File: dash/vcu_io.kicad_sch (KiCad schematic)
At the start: 56 parts, among them J3 M80-5102042, Q2 XP262N7002TR-G, Q3 XP262N7002TR-G, Q4 XP262N7002TR-G, Q5 XP262N7002TR-G, U30 TCAN3404-Q1, U42 TCAN3404-Q1

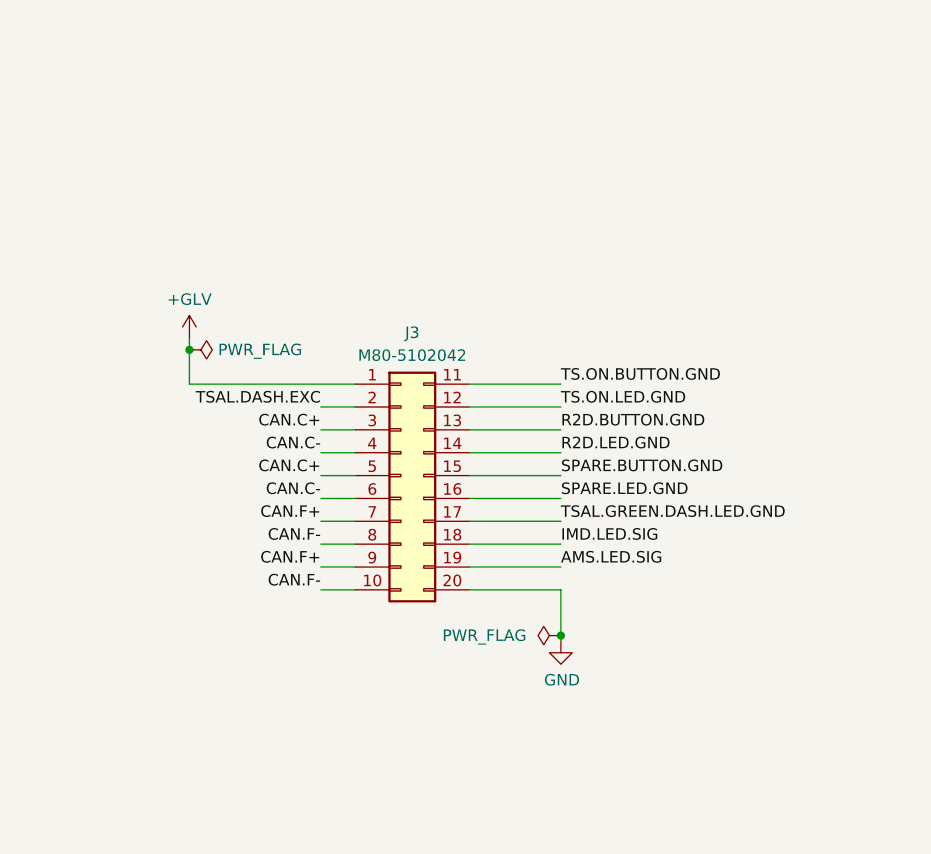
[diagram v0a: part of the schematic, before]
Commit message: Changed Inductors
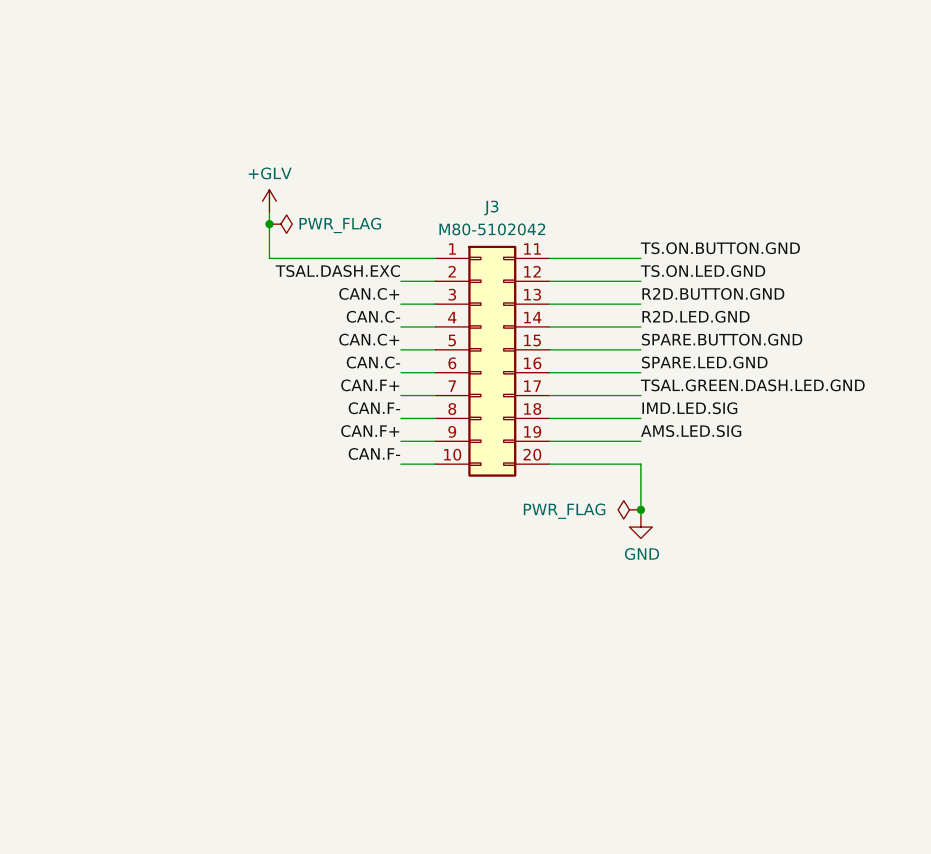
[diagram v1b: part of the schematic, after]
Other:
- moved on the sheet: J3

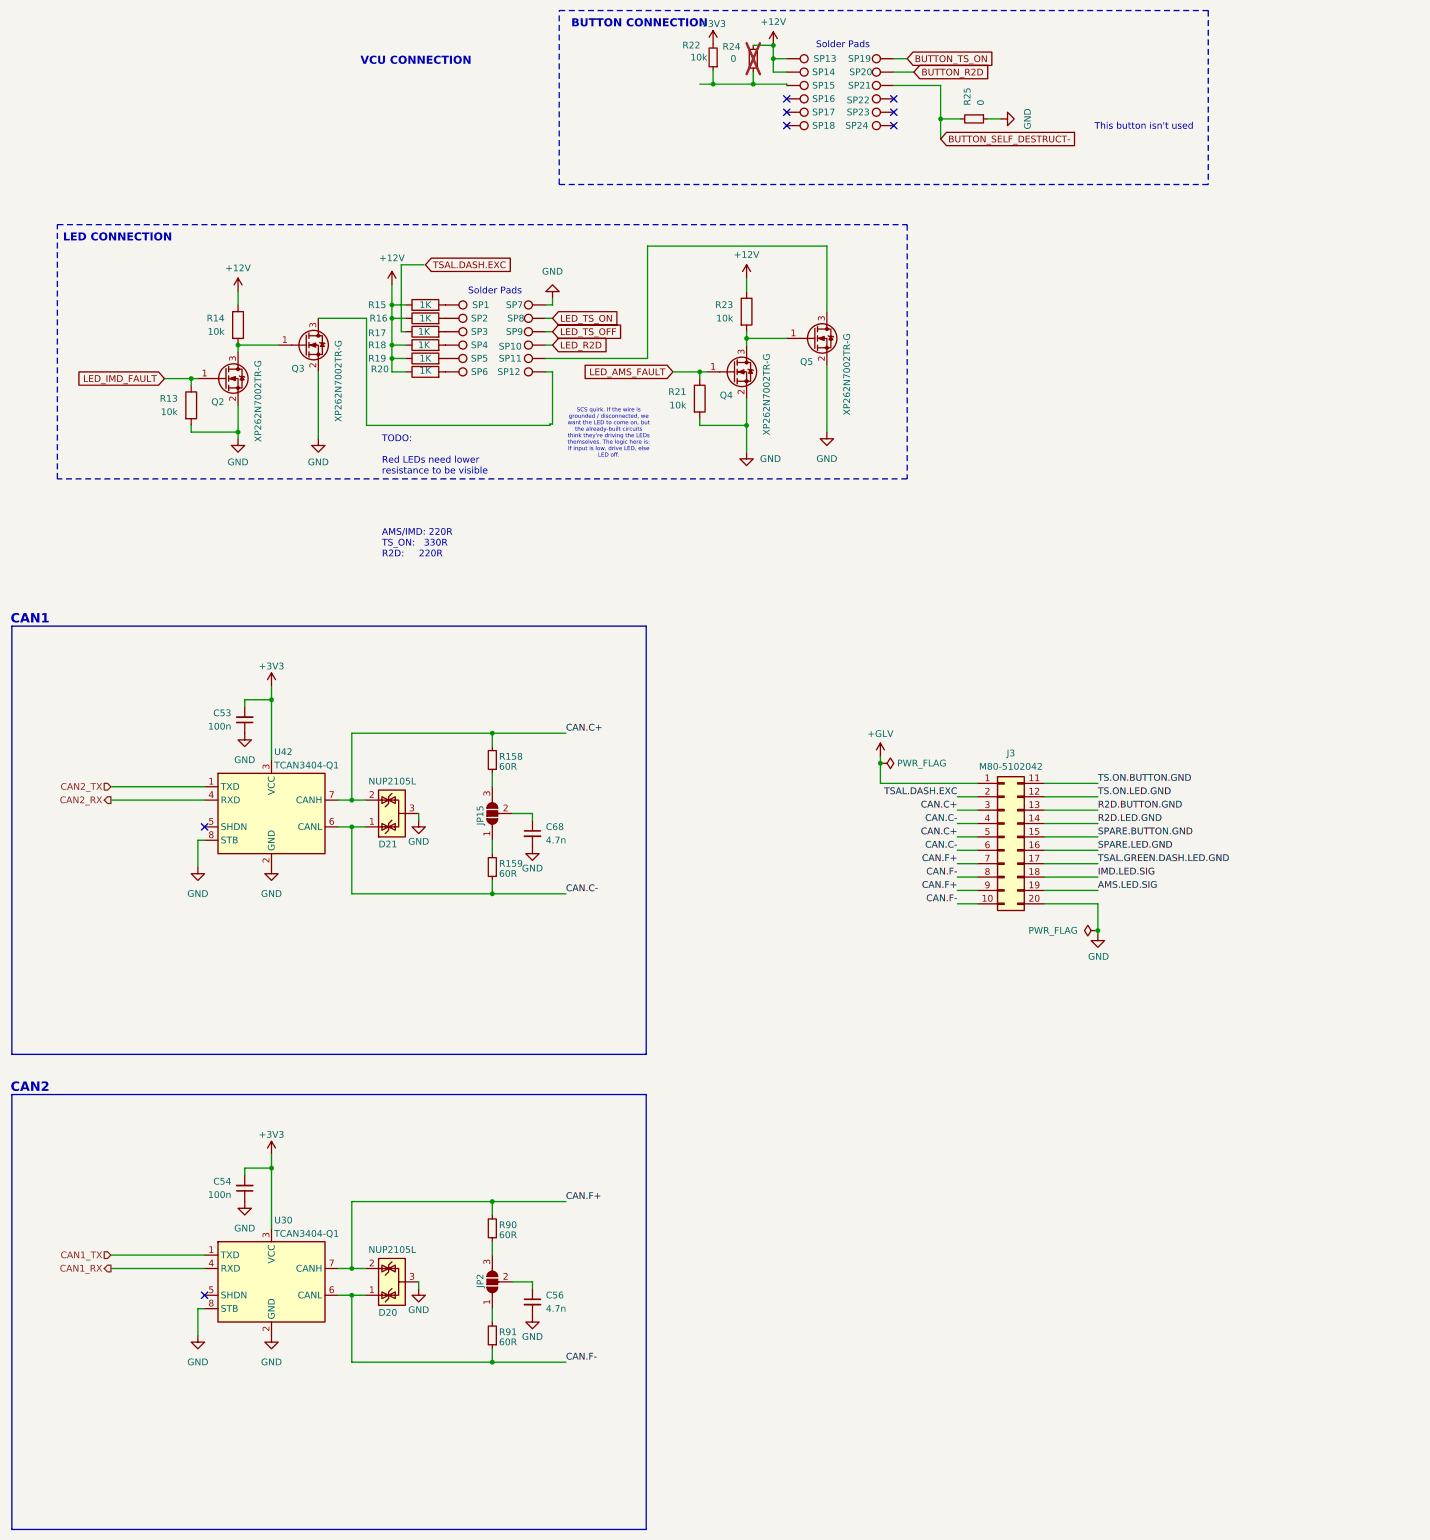
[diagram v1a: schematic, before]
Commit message: Beep Boop
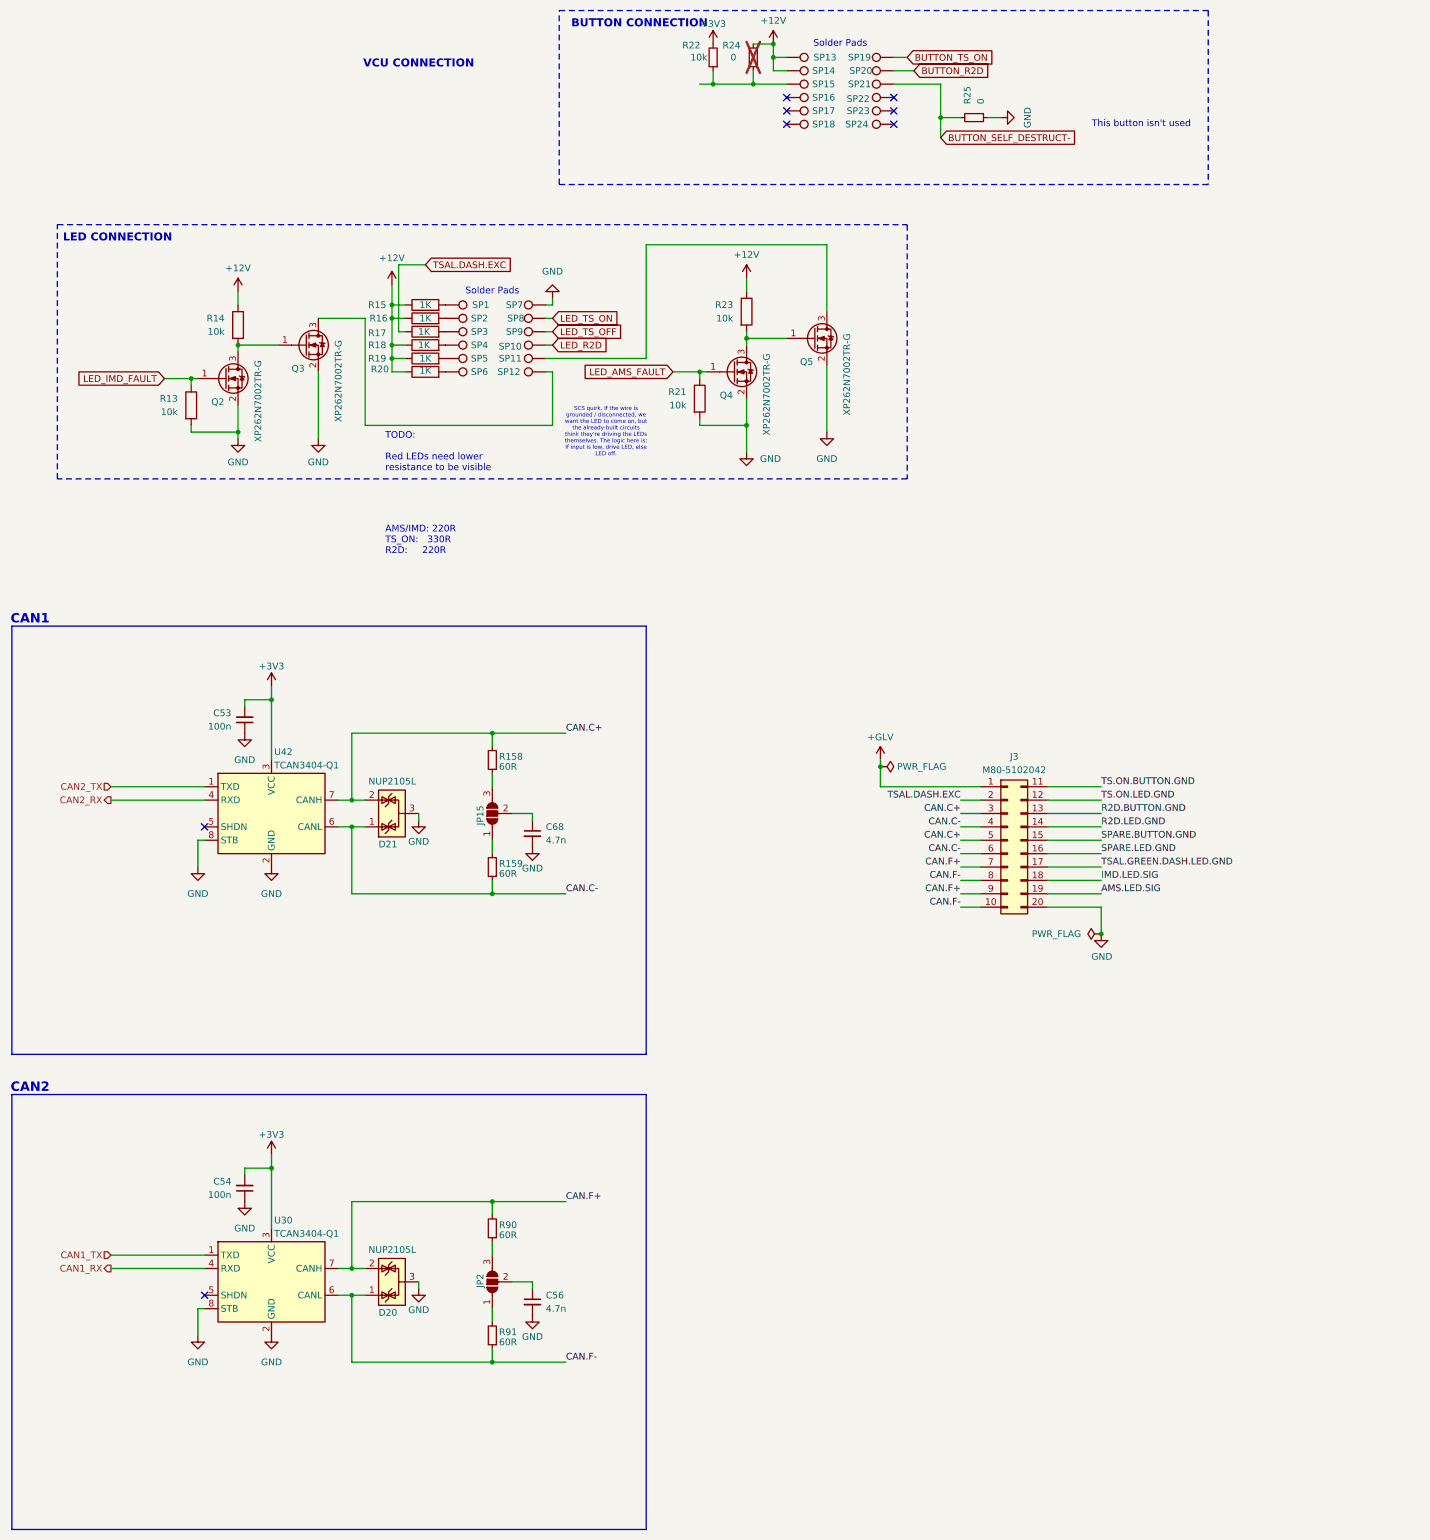
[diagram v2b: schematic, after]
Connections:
- net TSAL.DASH.EXC: now also R17.1
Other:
- moved on the sheet: J3

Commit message: Lots of routing stuff and updating connectors
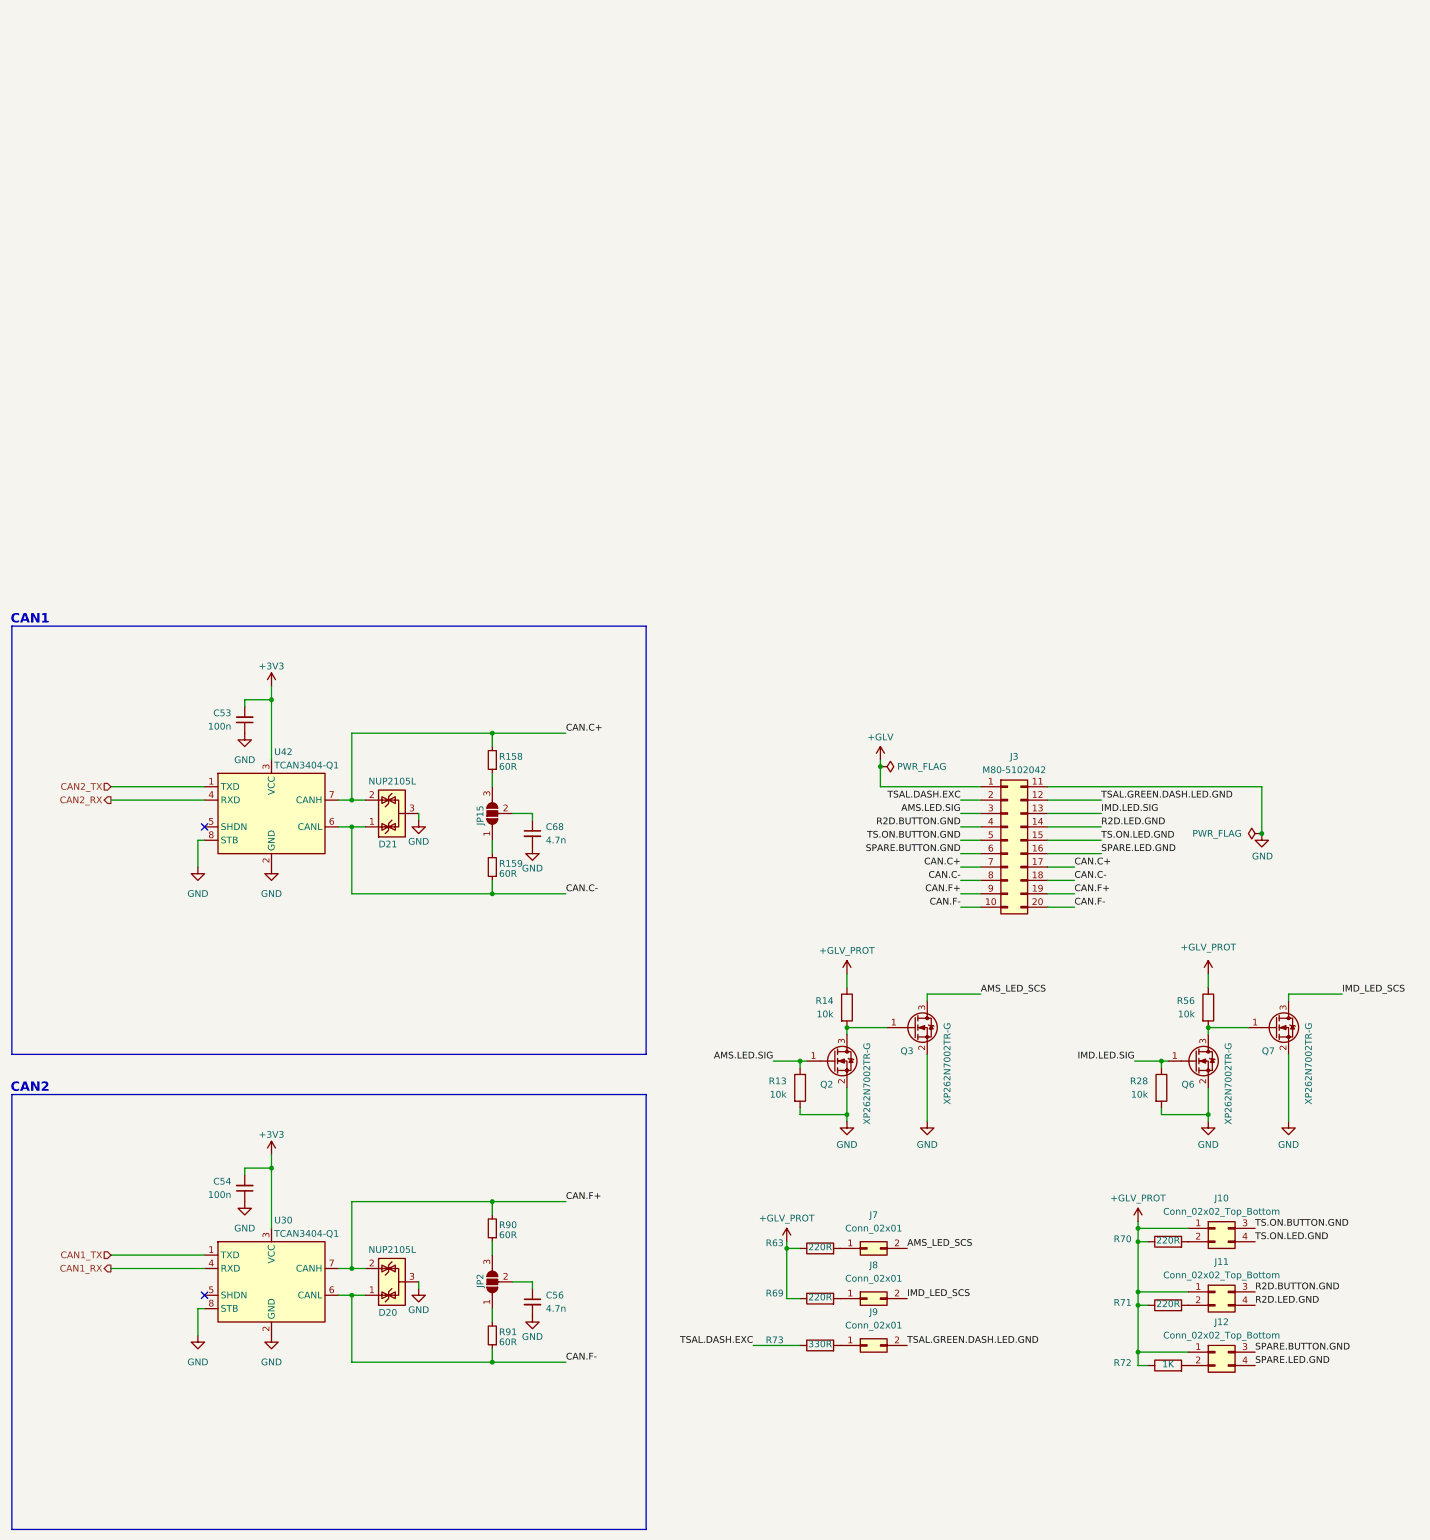
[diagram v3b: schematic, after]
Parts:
- removed Q4, Q5: XP262N7002TR-G, Package_TO_SOT_SMD:SOT-23, symbol Device:Q_NMOS_GSD
- removed R15, R16, R17, R18, R19, R20: 1K, Resistor_SMD:R_0603_1608Metric, symbol Device:R
- removed R21, R23: 10k, Resistor_SMD:R_0603_1608Metric, symbol Device:R
- removed R22: 10k, Resistor_SMD:R_0603_1608Metric, symbol Device:R_Small
- removed R24, R25: 0, Resistor_SMD:R_0603_1608Metric, symbol Device:R_Small
- removed SP1, SP10, SP11, SP12, SP13, SP14, SP15, SP16, SP17, SP18, SP19, SP2, SP20, SP21, SP22, SP23, SP24, SP3, SP4, SP5, SP6, SP7, SP8, SP9: Solder Pad, TestPoint:TestPoint_Pad_D2.0mm, symbol Connector:TestPoint
- added J10, J11, J12: Conn_02x02_Top_Bottom, Connector_Molex:Molex_Micro-Fit_3.0_43045-0412_2x02_P3.00mm_Vertical, symbol Connector_Generic:Conn_02x02_Top_Bottom
- added J7, J8, J9: Conn_02x01, Connector_Molex:Molex_Micro-Fit_3.0_43045-0212_2x01_P3.00mm_Vertical, symbol Connector_Generic:Conn_02x01
- added Q6, Q7: XP262N7002TR-G, Package_TO_SOT_SMD:SOT-23, symbol Device:Q_NMOS_GSD
- added R28, R56: 10k, Resistor_SMD:R_0603_1608Metric, symbol Device:R
- added R63, R69, R70, R71: 220R, Resistor_SMD:R_0603_1608Metric, symbol Device:R
- added R72: 1K, Resistor_SMD:R_0603_1608Metric, symbol Device:R
- added R73: 330R, Resistor_SMD:R_0603_1608Metric, symbol Device:R
- U30, U42: footprint Package_SO:SOIC-8_3.9x4.9mm_P1.27mm -> Package_TO_SOT_SMD:SOT-23-8_Handsoldering
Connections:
- net LED_IMD_FAULT is gone; now on net AMS.LED.SIG: Q2.1 (G), R13.1
- net AMS.LED.SIG: now also J3.3 (Pin_3); no longer J3.19 (Pin_19)
- net CAN.C+: now also J3.17 (Pin_17), J3.7 (Pin_7); no longer J3.3 (Pin_3), J3.5 (Pin_5)
- net CAN.C-: now also J3.18 (Pin_18), J3.8 (Pin_8); no longer J3.4 (Pin_4), J3.6 (Pin_6)
- net CAN.F+: now also J3.19 (Pin_19); no longer J3.7 (Pin_7)
- net CAN.F-: now also J3.20 (Pin_20); no longer J3.8 (Pin_8)
- net GND: now also J3.11 (Pin_11), Q6.2 (S), Q7.2 (S), R28.2; no longer J3.20 (Pin_20)
- net IMD.LED.SIG: now also J3.13 (Pin_13), Q6.1 (G), R28.1; no longer J3.18 (Pin_18)
- net R2D.BUTTON.GND: now also J3.4 (Pin_4), J11.3 (Pin_3); no longer J3.13 (Pin_13)
- net R2D.LED.GND: now also J11.4 (Pin_4)
- net SPARE.BUTTON.GND: now also J3.6 (Pin_6), J12.3 (Pin_3); no longer J3.15 (Pin_15)
- net SPARE.LED.GND: now also J12.4 (Pin_4)
- net TS.ON.BUTTON.GND: now also J3.5 (Pin_5), J10.3 (Pin_3); no longer J3.11 (Pin_11)
- net TS.ON.LED.GND: now also J3.15 (Pin_15), J10.4 (Pin_4); no longer J3.12 (Pin_12)
- net TSAL.DASH.EXC: now also R73.1
- net TSAL.GREEN.DASH.LED.GND: now also J3.12 (Pin_12), J9.2 (Pin_2); no longer J3.17 (Pin_17)
- net AMS_LED_SCS: now reaches Q3.3 (D)
- net AMS_LED_SCS: now also J7.2 (Pin_2)
- net +12V renamed +GLV_PROT
- net +GLV_PROT: now also J10.1 (Pin_1), J11.1 (Pin_1), J12.1 (Pin_1), R56.1, R63.1, R69.1, R70.1, R71.1, R72.1
- new net: J12.2 (Pin_2), R72.2
- new net: J10.2 (Pin_2), R70.2
- new net: J7.1 (Pin_1), R63.2
- new net: J8.1 (Pin_1), R69.2
- new net: J9.1 (Pin_1), R73.2
- new net: J11.2 (Pin_2), R71.2
- new net: Q6.3 (D), Q7.1 (G), R56.2
- new net IMD_LED_SCS: J8.2 (Pin_2), Q7.3 (D)
- no-connect marks 8 -> 2
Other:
- note removed: "AMS/IMD: 220R TS_ON: 330R R2D: 220R"
- note removed: "BUTTON CONNECTION"
- note removed: "LED CONNECTION"
- note removed: "SCS quirk. If the wire is grounded / disconnected, we want the LED to come on, but the already-built circuits think they're driving the LEDs themselves. The logic here is: If input is low, drive LED, else LED off."
- note removed: "Solder Pads"
- note removed: "TODO: Red LEDs need lower resistance to be visible"
- note removed: "This button isn't used"
- note removed: "VCU CONNECTION"
- moved on the sheet: Q2, Q3, R13, R14
